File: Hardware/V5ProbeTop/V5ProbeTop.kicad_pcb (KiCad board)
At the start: 2 copper layers, 126.4 x 15.2 mm, 8 parts

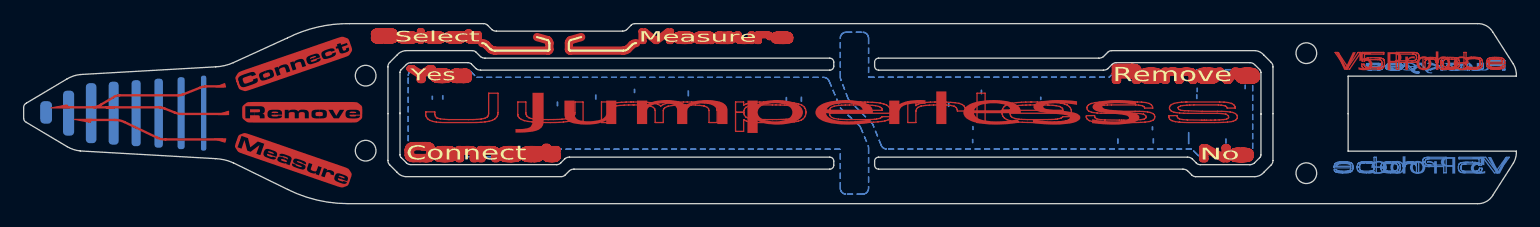
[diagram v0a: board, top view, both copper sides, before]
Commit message: routed V5r4
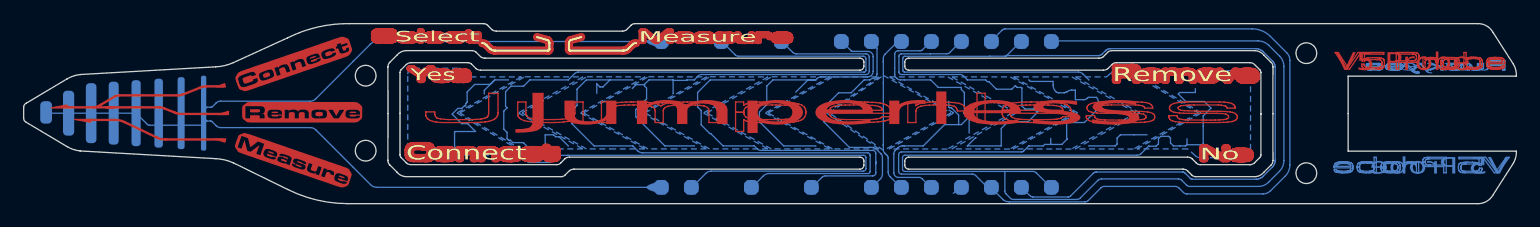
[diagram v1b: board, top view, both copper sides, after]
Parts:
- added J1: Conn_01x13_Socket, JumperlessFootprints:Probe_capsense_connect, B.Cu at (159.7, 92.4)
- added J2: Conn_01x13_Socket, JumperlessFootprints:Probe_capsense_connect, B.Cu at (159.7, 80.1)
- added TP1: TestPoint, JumperlessFootprints:Tiniest_Possible_pad, B.Cu at (114.2, 89.4)
- added TP10: TestPoint, JumperlessFootprints:Tiniest_Possible_pad, B.Cu at (152.6, 88.9)
- added TP11: TestPoint, JumperlessFootprints:Tiniest_Possible_pad, B.Cu at (157.8, 83.3)
- added TP12: TestPoint, JumperlessFootprints:Tiniest_Possible_pad, B.Cu at (162.8, 88.9)
- added TP13: TestPoint, JumperlessFootprints:Tiniest_Possible_pad, B.Cu at (167.9, 88.9)
- added TP14: TestPoint, JumperlessFootprints:Tiniest_Possible_pad, B.Cu at (87.9, 89.0)
- added TP15: TestPoint, JumperlessFootprints:Tiniest_Possible_pad, B.Cu at (113.7, 83.3)
- added TP16: TestPoint, JumperlessFootprints:Tiniest_Possible_pad, B.Cu at (118.8, 83.3)
- added TP17: TestPoint, JumperlessFootprints:Tiniest_Possible_pad, B.Cu at (124.2, 83.3)
- added TP18: TestPoint, JumperlessFootprints:Tiniest_Possible_pad, B.Cu at (129.4, 83.3)
- added TP19: TestPoint, JumperlessFootprints:Tiniest_Possible_pad, B.Cu at (134.5, 83.3)
- added TP2: TestPoint, JumperlessFootprints:Tiniest_Possible_pad, B.Cu at (118.8, 88.9)
- added TP20: TestPoint, JumperlessFootprints:Tiniest_Possible_pad, B.Cu at (139.7, 83.3)
- added TP21: TestPoint, JumperlessFootprints:Tiniest_Possible_pad, B.Cu at (144.3, 83.3)
- added TP22: TestPoint, JumperlessFootprints:Tiniest_Possible_pad, B.Cu at (145.4, 83.6)
- added TP23: TestPoint, JumperlessFootprints:Tiniest_Possible_pad, B.Cu at (147.2, 83.3)
- added TP24: TestPoint, JumperlessFootprints:Tiniest_Possible_pad, B.Cu at (152.6, 83.3)
- added TP25: TestPoint, JumperlessFootprints:Tiniest_Possible_pad, B.Cu at (157.8, 88.9)
- added TP26: TestPoint, JumperlessFootprints:Tiniest_Possible_pad, B.Cu at (162.8, 83.3)
- added TP27: TestPoint, JumperlessFootprints:Tiniest_Possible_pad, B.Cu at (167.8, 82.8)
- added TP28: TestPoint, JumperlessFootprints:Tiniest_Possible_pad, B.Cu at (87.9, 83.1)
- added TP3: TestPoint, JumperlessFootprints:Tiniest_Possible_pad, B.Cu at (124.2, 88.9)
- added TP4: TestPoint, JumperlessFootprints:Tiniest_Possible_pad, B.Cu at (129.4, 88.9)
- added TP5: TestPoint, JumperlessFootprints:Tiniest_Possible_pad, B.Cu at (134.5, 88.9)
- added TP6: TestPoint, JumperlessFootprints:Tiniest_Possible_pad, B.Cu at (139.7, 88.9)
- added TP7: TestPoint, JumperlessFootprints:Tiniest_Possible_pad, B.Cu at (144.3, 89.0)
- added TP8: TestPoint, JumperlessFootprints:Tiniest_Possible_pad, B.Cu at (145.4, 88.8)
- added TP9: TestPoint, JumperlessFootprints:Tiniest_Possible_pad, B.Cu at (147.2, 88.9)
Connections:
- REF** pad 1: (no net) -> Net-(J1-Pin_1)
- REF** pad 2: (no net) -> Net-(J1-Pin_1)
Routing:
- net Net-(J1-Pin_2): track 0.00 -> 106.8 mm
- net Net-(J1-Pin_4): track 0.00 -> 101.5 mm
- net Net-(J1-Pin_1): track 0.00 -> 97.6 mm
- net Net-(J1-Pin_3): track 0.00 -> 88.6 mm
- net Net-(J1-Pin_14): track 0.00 -> 65.9 mm
- net Net-(J1-Pin_13): track 0.00 -> 56.7 mm
- net Net-(J1-Pin_12): track 0.00 -> 49.4 mm
- net Net-(J1-Pin_11): track 0.00 -> 40.3 mm
- net Net-(J1-Pin_5): track 0.00 -> 33.5 mm
- net Net-(J1-Pin_10): track 0.00 -> 32.1 mm
- net Net-(J1-Pin_6): track 0.00 -> 31.0 mm
- net Net-(J1-Pin_9): track 0.00 -> 25.1 mm
- net Net-(J1-Pin_8): track 0.00 -> 19.2 mm
- net Net-(J1-Pin_7): track 0.00 -> 13.9 mm
- net (no net): track 6.98 -> 0.00 mm
- added copper zone on B.Cu, net Net-(J1-Pin_10)
- added copper zone on B.Cu, net Net-(J1-Pin_11)
- added copper zone on B.Cu, net Net-(J1-Pin_12)
- added copper zone on B.Cu, net Net-(J1-Pin_13)
- added copper zone on B.Cu, net Net-(J1-Pin_14)
- added copper zone on B.Cu, net Net-(J1-Pin_2)
- added copper zone on B.Cu, net Net-(J1-Pin_3)
- added copper zone on B.Cu, net Net-(J1-Pin_4)
- added copper zone on B.Cu, net Net-(J1-Pin_5)
- added copper zone on B.Cu, net Net-(J1-Pin_6)
- added copper zone on B.Cu, net Net-(J1-Pin_7)
- added copper zone on B.Cu, net Net-(J1-Pin_8)
- added copper zone on B.Cu, net Net-(J1-Pin_9)
- removed copper zone on B.Cu, net (none)
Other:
- outline, holes or cut-outs redrawn
